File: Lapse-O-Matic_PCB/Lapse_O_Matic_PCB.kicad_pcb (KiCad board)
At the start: 2 copper layers, 39.9 x 79.9 mm, 38 parts, among them J1 PIR, J10 POWER, J11 LOGO4, J2 TRIG, J3 RTC_DS3231, J4 PROG, J5 PROG_EN, J6 LOGO1, J7 LOGO2, J8 PCB, J9 LOGO3, Q1 2N3904, Q2 2N3904, Q3 BD135, SW1 POWER, SW2 TRIGGER, U1 MCP1826S-3302, U3 ESP32_CAM

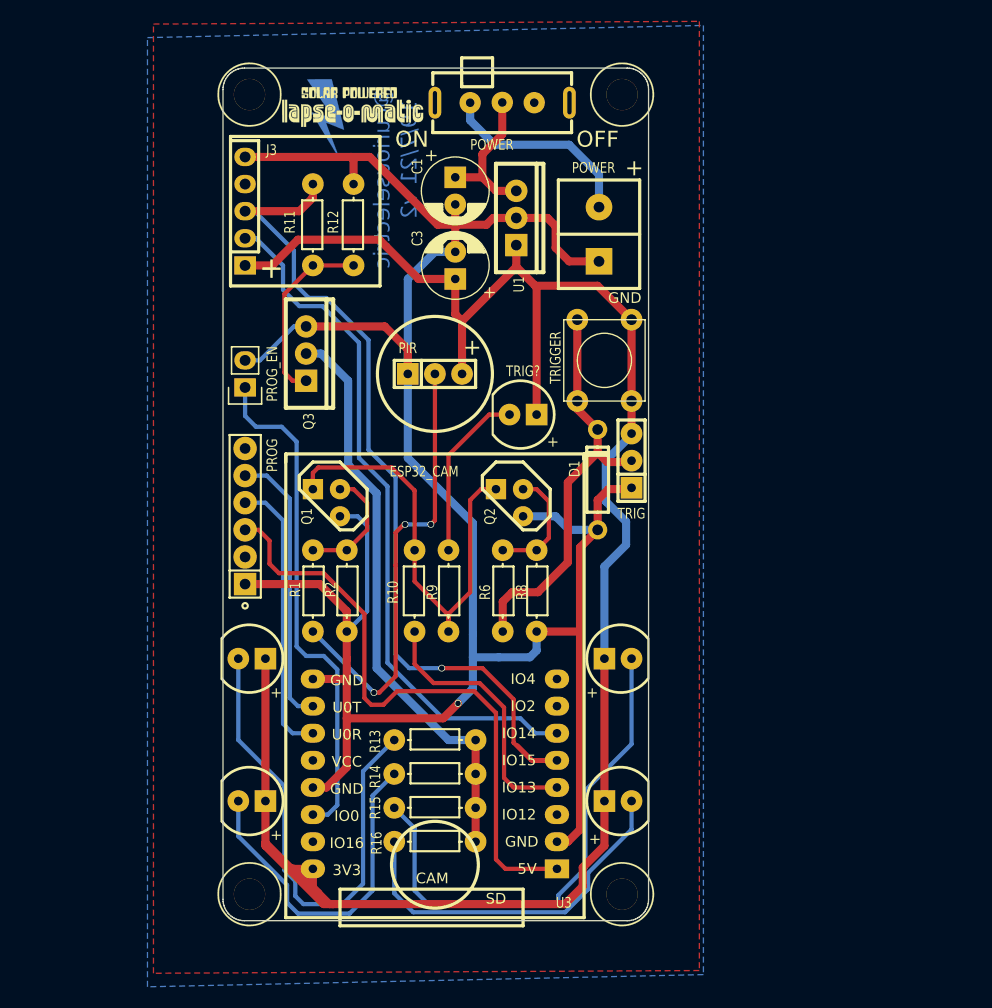
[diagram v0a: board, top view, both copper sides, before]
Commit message: updated PCB and hardware
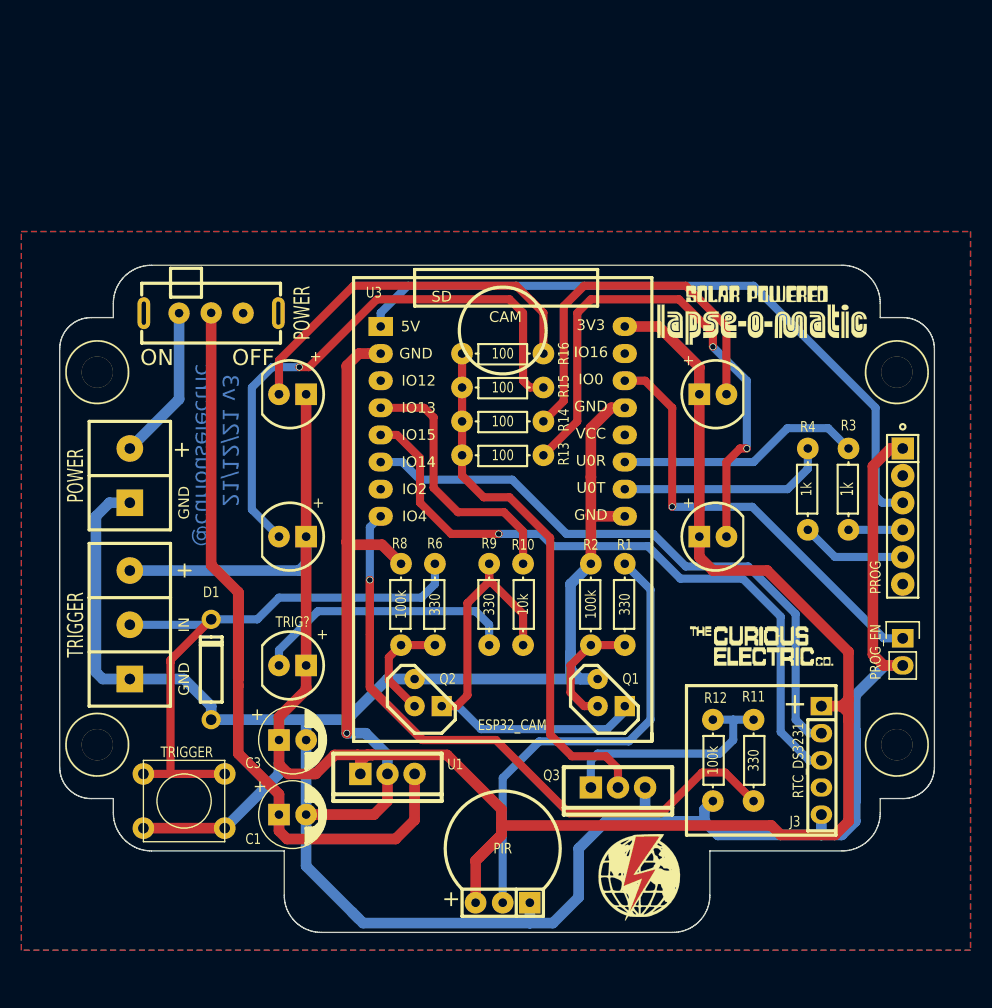
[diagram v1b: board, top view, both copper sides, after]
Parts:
- added R3: 1k, REInnovationFootprint:TH_Resistor_1, F.Cu at (158.8, 86.4)
- added R4: 1k, REInnovationFootprint:TH_Resistor_1, F.Cu at (154.9, 86.4)
- J2: value TRIG -> TRIGGER; footprint REInnovationFootprint:SIL-3_lg_pad -> REInnovationFootprint:SIL-3_screw_terminal
- J6: moved to F.Cu
- J7: moved to B.Cu
- J8: footprint REInnovationFootprint:PCB_SolarChargerPCB40x80 -> REInnovationFootprint:PCB_Lapse-O-Matic
- J9: footprint REInnovationGraphics:lapseomatic logo -> REInnovationGraphics:lapseomatic logo_20x6mm
- Q1, Q2: value 2N3904 -> BC547C
- R1, R11, R6: value 1k -> 330
- R12, R2, R8: value 10k -> 100k
- moved J7 77.1 mm to (139.8, 126.7), turned to 180 degrees
- moved J3 71.5 mm to (143.6, 118.8), turned to 0 degrees
- moved J5 65.9 mm to (163.8, 100.3), turned to 0 degrees
- moved R11 65.0 mm to (149.9, 111.8), turned to 270 degrees
- moved J4 61.6 mm to (163.8, 88.9), turned to 270 degrees
- moved R12 60.4 mm to (146.1, 111.8), turned to 270 degrees
- moved C1 60.4 mm to (106.7, 116.8), turned to 0 degrees
- moved D6 57.6 mm to (146.1, 77.5), turned to 0 degrees
- moved SW2 57.0 mm to (96.5, 115.6), turned to 0 degrees
- moved U1 53.4 mm to (115.6, 113.0), turned to 270 degrees
- moved J2 51.2 mm to (91.4, 104.1)
- moved U3 51.2 mm to (126.4, 71.1), turned to 0 degrees
- moved Q3 50.0 mm to (137.2, 114.3), turned to 270 degrees
- moved J10 49.4 mm to (91.4, 87.6)
- moved D8 48.8 mm to (106.7, 77.5), turned to 180 degrees
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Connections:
- J4 pad 4: /U0R -> Net-(J4-Pad4)
- J4 pad 5: /U0T -> Net-(J4-Pad5)
- R11 pad 2: /I2C_CLK -> /FLASH
- U3 pad 8: Net-(U3-Pad8) -> /FLASH
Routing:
- net /FLASH: track 0.00 -> 83.9 mm, vias 0 -> 1
- net GND: track 228.5 -> 302.2 mm
- net Net-(C1-Pad1): track 14.0 -> 77.3 mm
- net Net-(D1-Pad1): track 38.6 -> 73.9 mm
- net +3V3: track 185.5 -> 212.3 mm
- net /I2C_CLK: track 82.9 -> 62.7 mm
- net Net-(J4-Pad5): track 0.00 -> 9.94 mm
- net Net-(D4-Pad2): track 16.2 -> 25.1 mm
- net /I2C_DAT: track 65.7 -> 58.5 mm
- net /5V_PWR: track 57.3 -> 64.5 mm
- net /U0T: track 26.2 -> 19.8 mm
- net /PROG_EN: track 47.7 -> 41.5 mm, vias 0 -> 1
- net Net-(Q3-Pad1): track 17.3 -> 22.4 mm
- net Net-(J4-Pad4): track 0.00 -> 5.08 mm
- net Net-(D7-Pad2): track 48.2 -> 52.9 mm, vias 0 -> 1
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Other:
- board size 39.9 x 79.9 mm -> 81.9 x 62.5 mm
- board text added: "21/12/21 v3"
- board text removed: "19/7/21 v2"
